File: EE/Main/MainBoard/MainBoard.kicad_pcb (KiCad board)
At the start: 2 copper layers, 185.6 x 109.5 mm, 18 parts, among them J1 Conn_02x13_Odd_Even

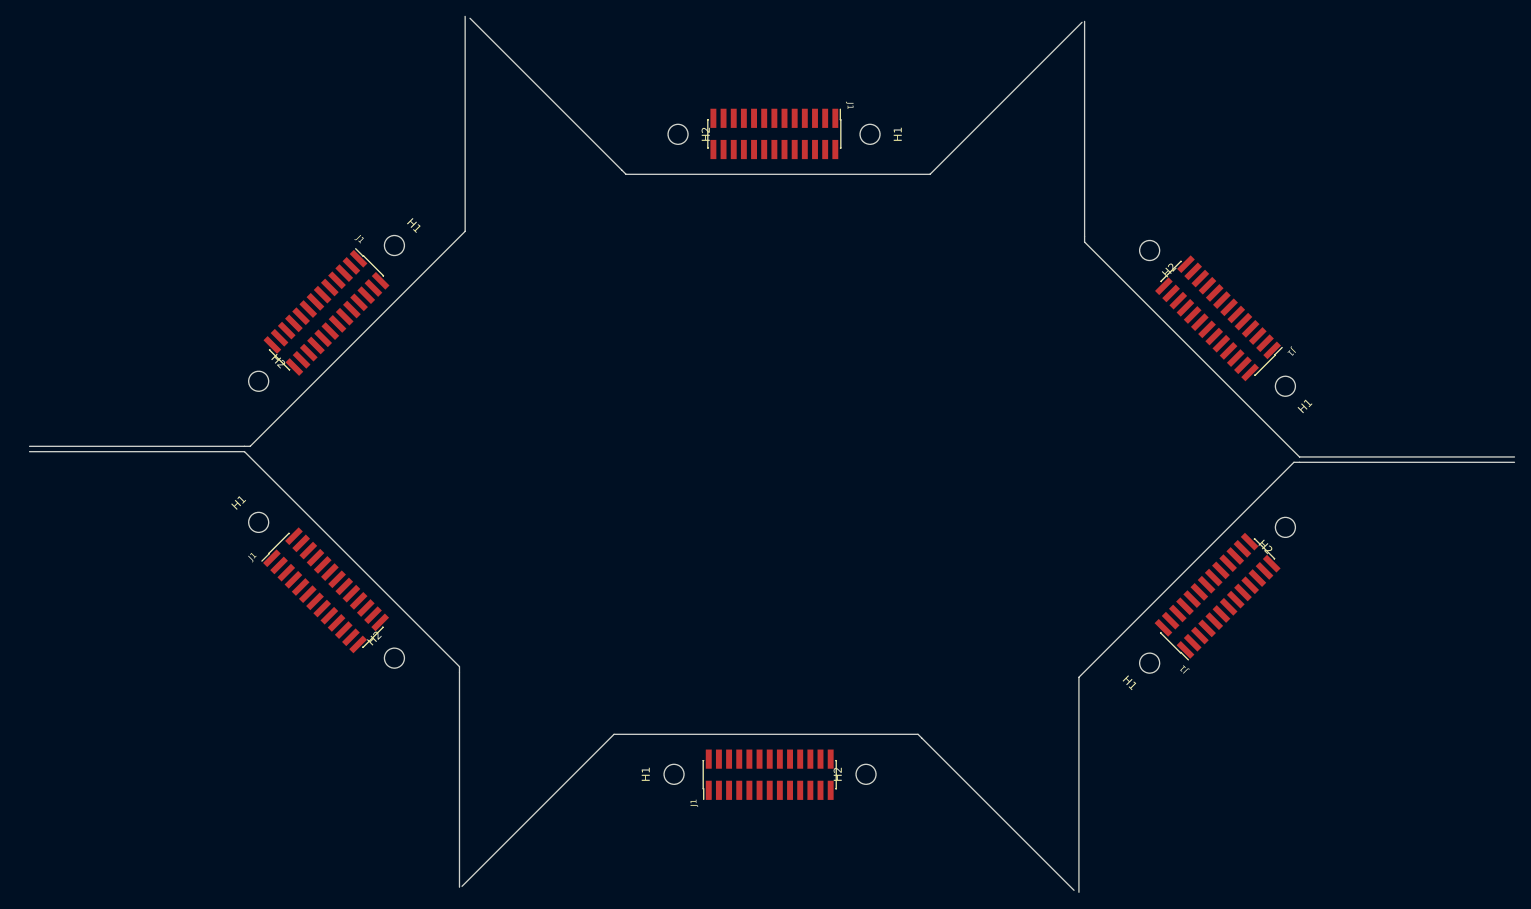
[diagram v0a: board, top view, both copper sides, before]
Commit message: First pass exterior
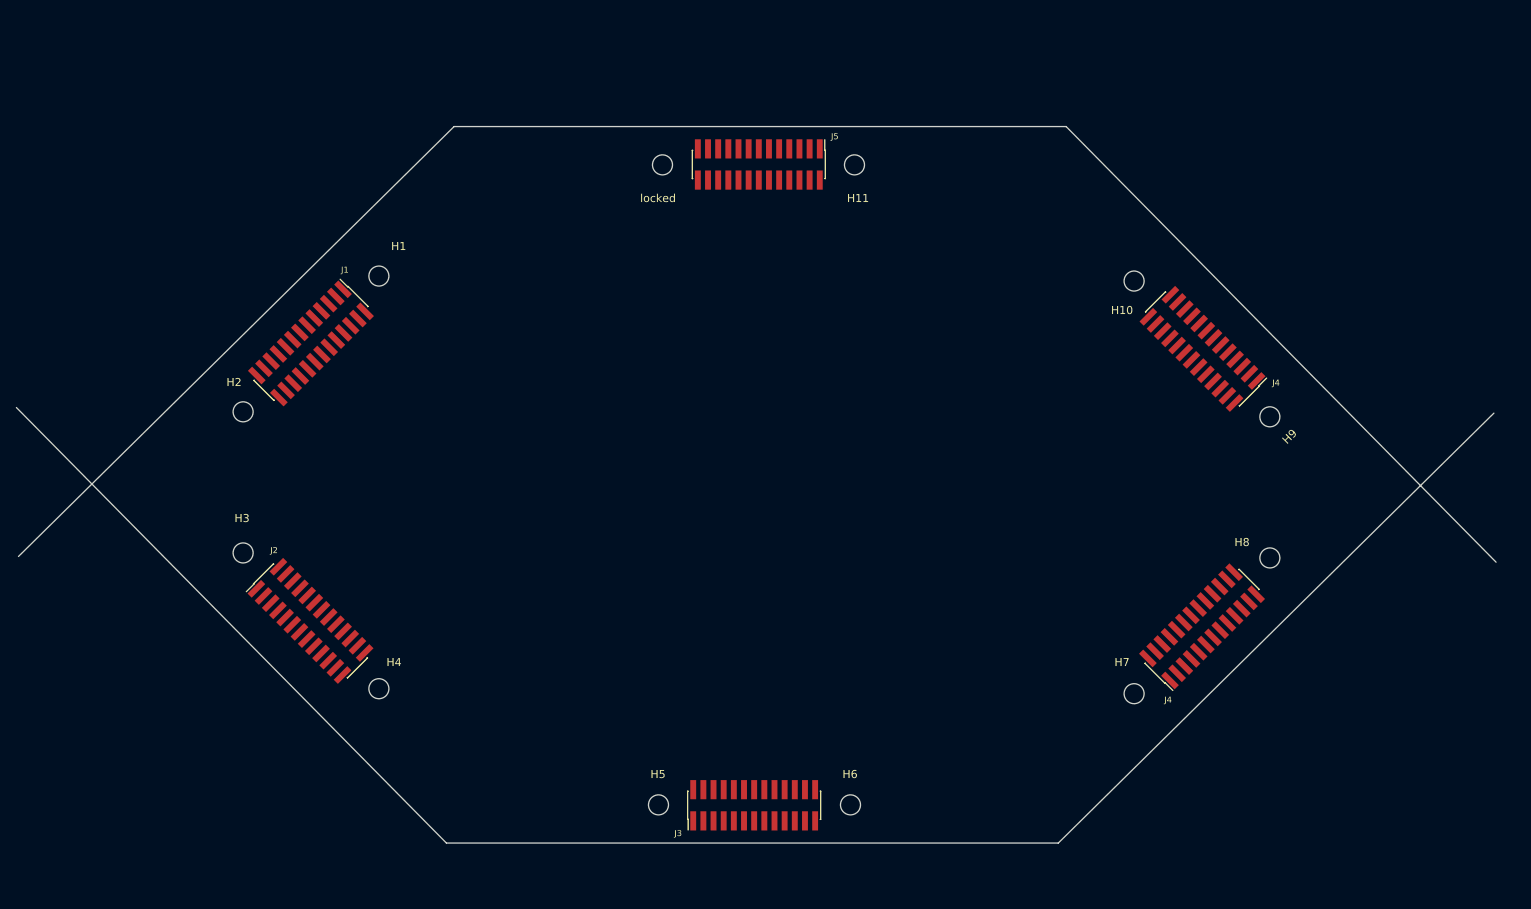
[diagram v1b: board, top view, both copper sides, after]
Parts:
- moved H5 4.29 mm to (131.1, 134.8)
- moved H6 4.29 mm to (155.1, 134.8)
- moved H1 4.29 mm to (96.1, 68.7)
- moved H10 4.29 mm to (190.5, 69.3)
- moved H11 4.29 mm to (155.6, 54.8)
- moved H2 4.29 mm to (79.1, 85.7)
- moved H3 4.29 mm to (79.1, 103.3)
- moved H4 4.29 mm to (96.1, 120.3)
- moved H7 4.29 mm to (190.5, 120.9)
- moved H8 4.29 mm to (207.5, 104.0)
- moved H9 4.29 mm to (207.5, 86.3)
- moved J4 4.29 mm to (199.1, 77.8)
- moved J4 4.29 mm to (199.0, 112.5)
- moved locked 4.29 mm to (131.6, 54.8)
- moved J1 4.29 mm to (87.6, 77.1)
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- renumbered H2 to H10, H1 to H11, H1 to H3, H2 to H4, H1 to H5, H2 to H6, H1 to H7, H2 to H8, H1 to H9, J1 to J2, J1 to J3, J1 to J4, J1 to J5, H2 to locked
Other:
- board size 185.6 x 109.5 mm -> 185 x 89.6 mm
